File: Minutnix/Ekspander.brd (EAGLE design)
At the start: 222.3 x 21.9 mm, 14 parts, among them X1 FH12-12S-0.5S_THINNER, X6 JST-XH-03-PIN-LONG-PAD

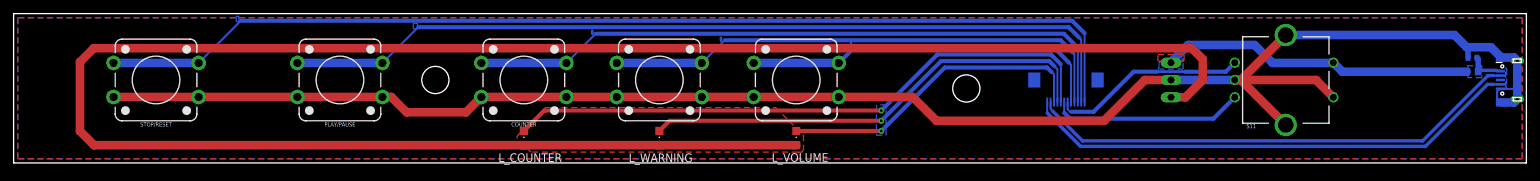
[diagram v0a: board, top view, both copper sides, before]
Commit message: Many final changes
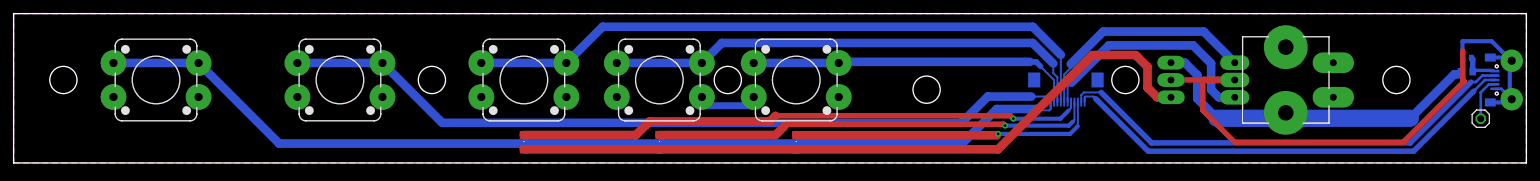
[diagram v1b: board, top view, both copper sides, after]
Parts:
- removed S11: ENCODER-SWITCH, SparkFun-Switches:ROTARY_ENC_PLAIN
- added ENCODER: ENCODER-SWITCH, MySparkFun-Switches:ROTARY_ENC_PLAIN
- added JP1: (no value), pinhead:1X01
- COUNTER, STOP/RESET, VOLUME, WARNING: device SparkFun-Switches:TACTILE_SWITCH_PTH_12MM -> MySparkFun-Switches:TACTILE_SWITCH_PTH_12MM
- moved C4 0.81 mm to (213.6, -6.50)
- moved L1 0.81 mm to (213.6, -8.53)
- moved U$1 0.81 mm to (220.5, -9.75)
- moved L_COUNTER 0.61 mm to (75.0, -18.9)
- moved L_VOLUME 0.61 mm to (115.0, -18.9)
- moved L_WARNING 0.61 mm to (94.9, -18.9)
- renumbered X1 to FFC_CON, X6 to POWER_CON
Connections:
- removed net N$1: FFC_CON.7, S11.A
- removed net N$10: FFC_CON.5, L_COUNTER.C
- removed net N$11: FFC_CON.4, L_WARNING.C
- removed net N$12: FFC_CON.3, L_VOLUME.C
- removed net N$17: FFC_CON.1, U$1.4
- removed net N$18: FFC_CON.2, U$1.2
- removed net N$2: FFC_CON.12, STOP/RESET.1, STOP/RESET.2
- removed net N$3: FFC_CON.11, PLAY/PAUSE.1, PLAY/PAUSE.2
- removed net N$4: COUNTER.1, COUNTER.2, FFC_CON.10
- removed net N$5: FFC_CON.9, WARNING.1, WARNING.2
- removed net N$6: FFC_CON.8, VOLUME.1, VOLUME.2
- removed net N$7: FFC_CON.6, S11.B
- new net COUNTER: COUNTER.1, COUNTER.2, FFC_CON.5
- new net DM: FFC_CON.11, U$1.2
- new net DP: FFC_CON.12, U$1.3
- new net ENC_A: ENCODER.A, FFC_CON.6
- new net ENC_B: ENCODER.B, FFC_CON.7
- new net L_COUNTER: FFC_CON.8, L_COUNTER.C
- new net L_VOLUME: FFC_CON.10, L_VOLUME.C
- new net L_WARNING: FFC_CON.9, L_WARNING.C
- new net N$8: JP1.1, U$1.4
- new net PLAY/PAUSE: FFC_CON.1, PLAY/PAUSE.1, PLAY/PAUSE.2
- new net STOP/RESET: FFC_CON.2, STOP/RESET.1, STOP/RESET.2
- new net VOLUME: FFC_CON.3, VOLUME.1, VOLUME.2
- new net WARNING: FFC_CON.4, WARNING.1, WARNING.2
- net +5V: now also ENCODER.P$3; no longer S11.SW-
- net GND: now also ENCODER.C; no longer FFC_CON.CASE1, FFC_CON.CASE2, S11.C, S11.P$3, S11.P$4, S11.SW+
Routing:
- net VCC: track 291.6 -> 105.2 mm
- net GND: track 256.2 -> 99.1 mm
- net N$2: track 156.2 -> 0.00 mm
- net STOP/RESET: track 0.00 -> 146.9 mm
- net N$3: track 127.3 -> 0.00 mm
- net PLAY/PAUSE: track 0.00 -> 116.2 mm
- net N$4: track 98.3 -> 0.00 mm
- net COUNTER: track 0.00 -> 96.0 mm
- net N$10: track 89.7 -> 0.00 mm, vias 1 -> 0
- net L_COUNTER: track 0.00 -> 83.3 mm, vias 0 -> 1
- net N$5: track 76.5 -> 0.00 mm
- net N$17: track 74.0 -> 0.00 mm
- net N$18: track 73.0 -> 0.00 mm
- net WARNING: track 0.00 -> 72.5 mm
- net DM: track 0.00 -> 69.1 mm
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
